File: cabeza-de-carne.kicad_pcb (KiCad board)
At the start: 2 copper layers, 28.2 x 29.7 mm, 20 parts, among them J1 Stomp_Connector, J2 Power_Connector, Q1 2N3904, Q2 BC182L

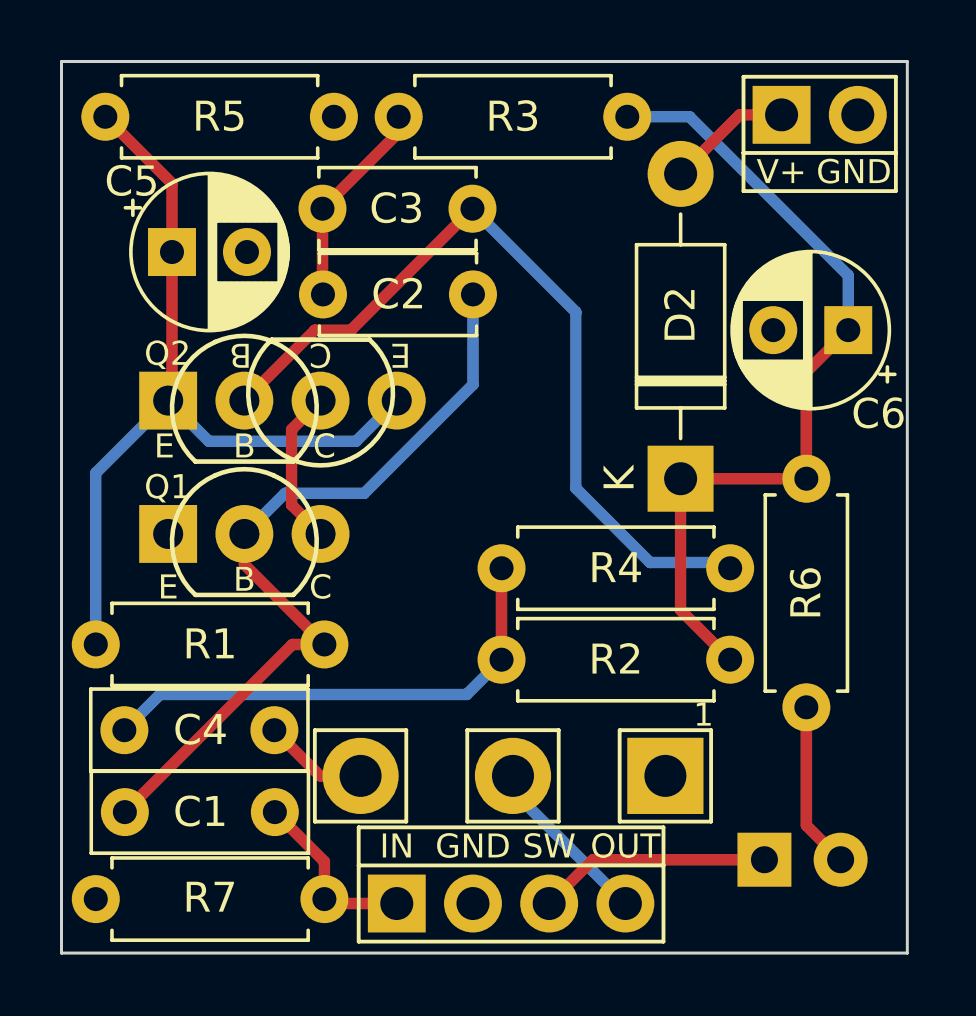
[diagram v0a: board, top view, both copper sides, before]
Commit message: 0.2: more compact board
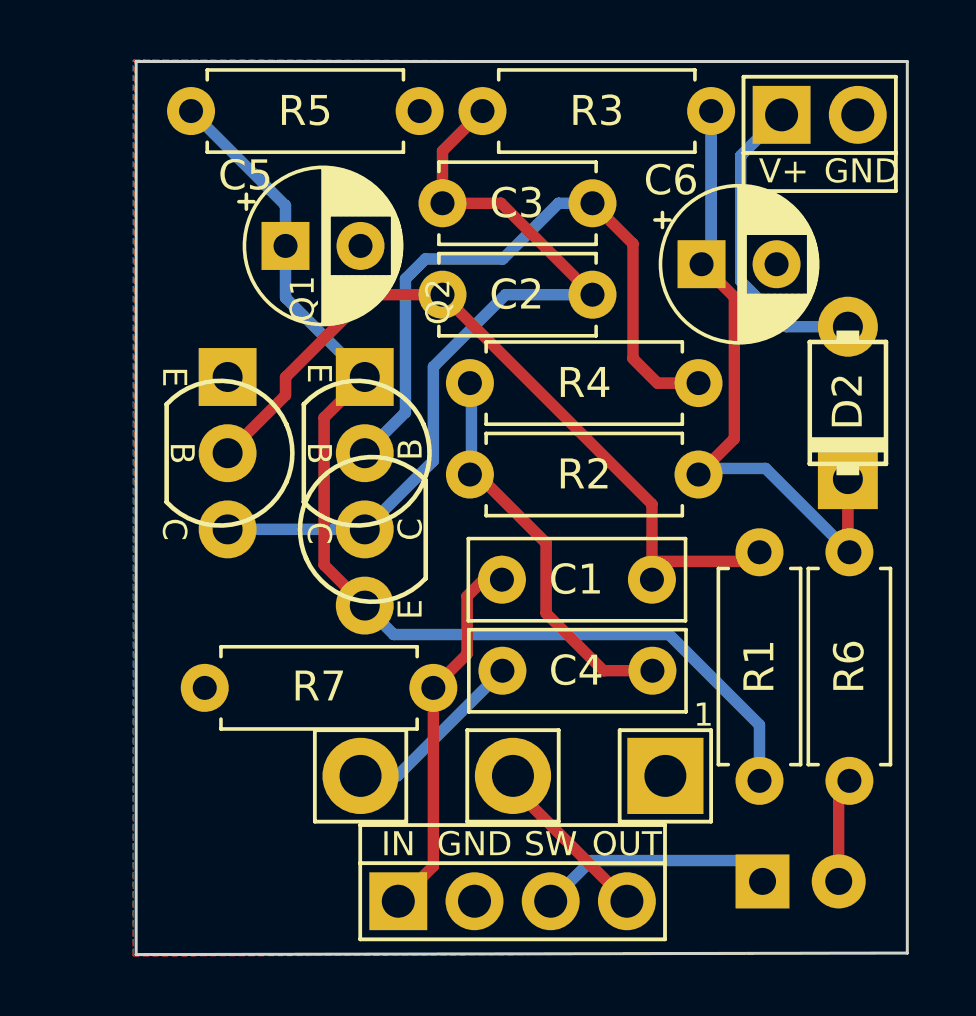
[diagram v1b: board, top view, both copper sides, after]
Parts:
- D1: footprint LED_THT:LED_D5.0mm -> LED_THT:LED_D3.0mm
- D2: footprint Diode_THT:D_DO-41_SOD81_P10.16mm_Horizontal -> diodes:DO41-2
- moved C4 17.7 mm to (242.2, -33.8), turned to 180 degrees
- moved R1 14.8 mm to (245.8, -37.7), turned to -90 degrees
- moved C1 10.8 mm to (237.2, -36.8), turned to 0 degrees
- moved R7 7.92 mm to (234.9, -33.2)
- moved R4 6.26 mm to (236.1, -43.4)
- moved R2 6.26 mm to (243.7, -40.3)
- moved D2 6.12 mm to (248.7, -42.7)
- moved C6 5.36 mm to (243.8, -47.3), turned to 0 degrees
- moved Q2 4.38 mm to (232.6, -41.0), turned to -90 degrees
- moved C3 4.00 mm to (235.2, -49.4)
- moved C5 3.79 mm to (230.0, -48.0)
- moved R5 2.86 mm to (226.8, -52.5)
- moved R6 2.84 mm to (248.8, -30.1)
- moved R3 2.80 mm to (244.2, -52.5)
- moved Q1 2.75 mm to (228.0, -41.0), turned to -90 degrees
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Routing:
- net Net-(C2-Pad2): track 12.2 -> 27.1 mm
- net Net-(C5-Pad1): track 28.3 -> 36.7 mm
- net IN: track 6.06 -> 12.8 mm
- net +9V: track 4.18 -> 10.3 mm
- net Net-(C6-Pad1): track 27.8 -> 21.8 mm
- net Net-(C3-Pad2): track 27.2 -> 21.9 mm
- net Net-(C4-Pad1): track 16.6 -> 13.0 mm
- net Net-(C4-Pad2): track 3.51 -> 6.18 mm
- net Net-(D1-Pad2): track 5.55 -> 3.50 mm
- net Net-(C1-Pad2): track 26.5 -> 25.2 mm
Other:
- board size 28.2 x 29.7 mm -> 25.7 x 29.8 mm
- board text added: "v0.2 2020-03-13"
- board text removed: "v0.1 2020-03-12"
